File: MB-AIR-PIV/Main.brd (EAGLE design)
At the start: 50.8 x 32.7 mm, 24 parts, among them IC1 MEGA8-AI, IC2 LM1117DTX-5.0, Y1 16MHZ

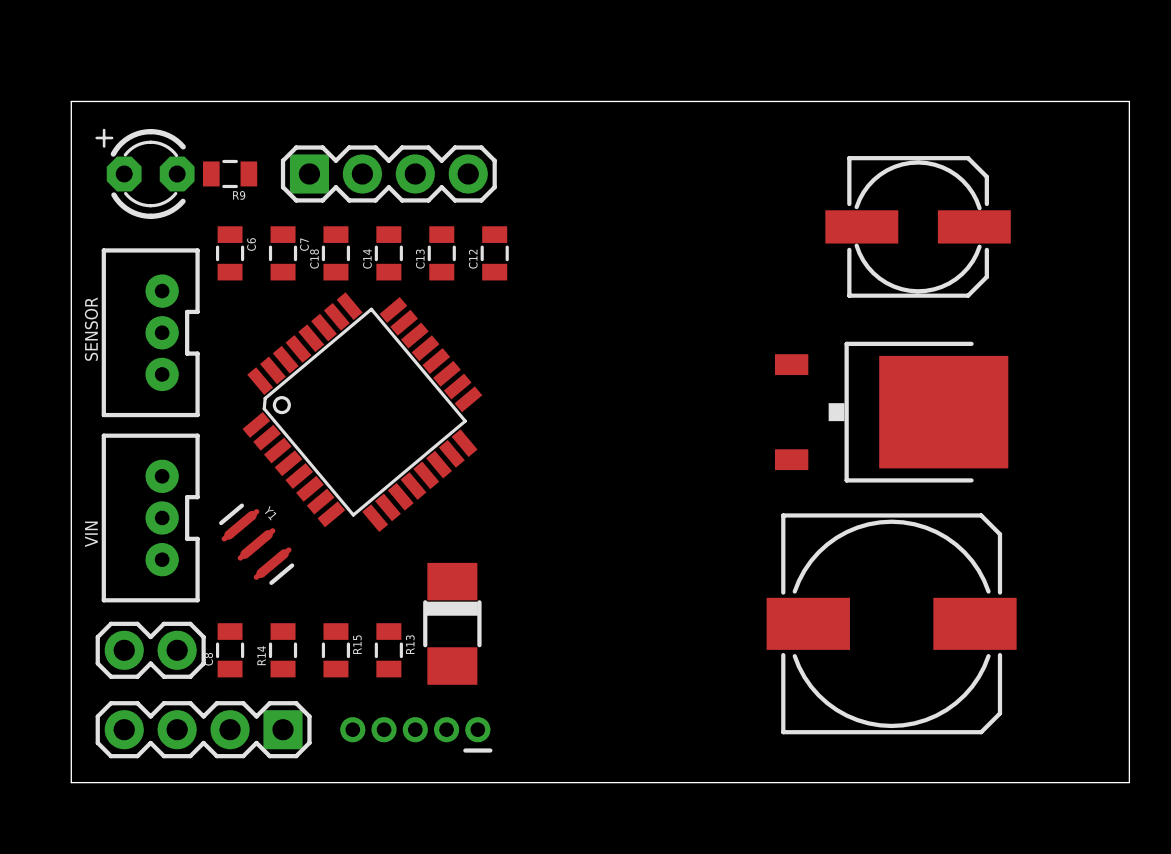
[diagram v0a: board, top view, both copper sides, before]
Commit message: update
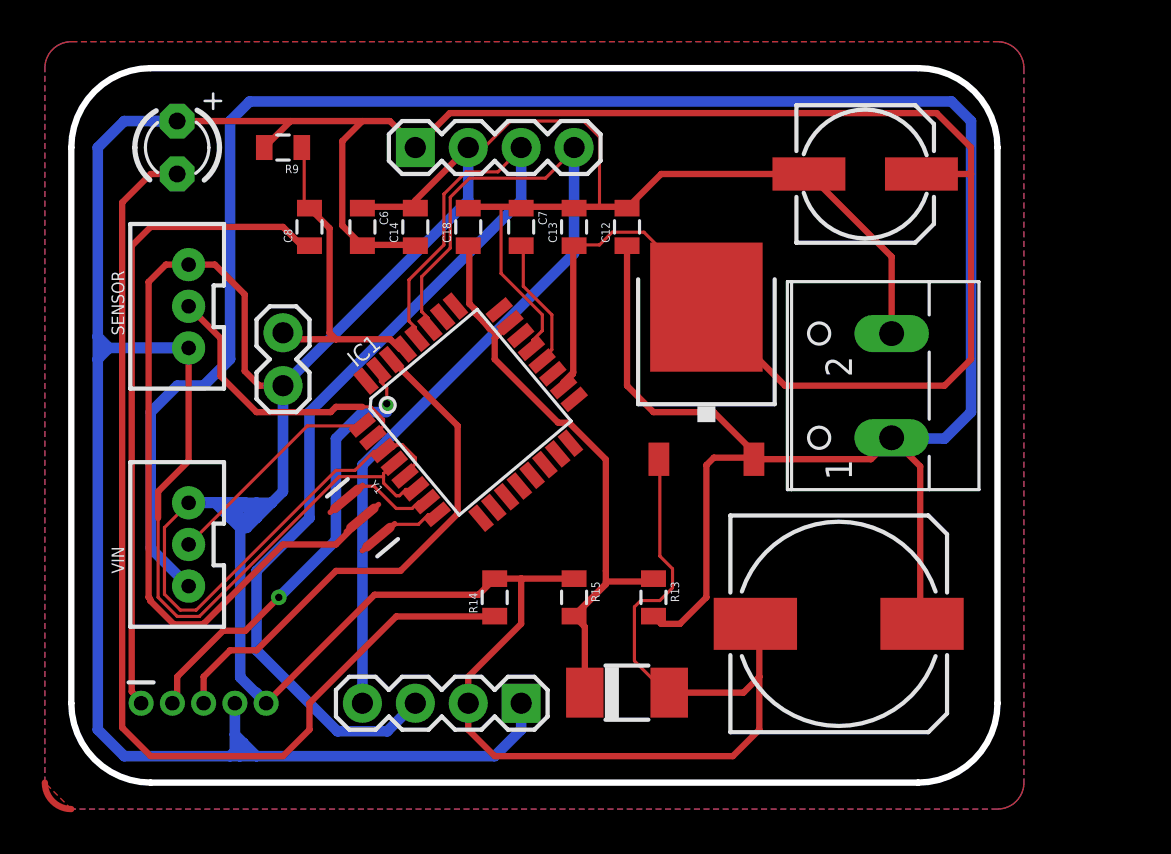
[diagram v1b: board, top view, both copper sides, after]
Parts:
- added X3: RELAY1, con-wago-500:W237-102
- moved C8 20.7 mm to (11.4, 26.7)
- moved JP1 17.0 mm to (10.2, 21.6), turned to 270 degrees
- moved R13 13.0 mm to (27.9, 8.89)
- moved R15 11.7 mm to (24.1, 8.89)
- moved BME280 11.5 mm to (21.6, 3.81)
- moved C7 11.5 mm to (21.6, 26.7)
- moved R14 10.5 mm to (20.3, 8.89)
- moved UPLOAD 10.2 mm to (6.35, 3.81), turned to 0 degrees
- moved IC2 9.25 mm to (30.5, 20.3), turned to 0 degrees
- moved D4 9.01 mm to (26.7, 4.32), turned to 0 degrees
- moved C12 6.48 mm to (26.7, 26.7)
- moved C18 6.48 mm to (19.1, 26.7)
- moved C6 6.48 mm to (14.0, 26.7)
- moved C13 6.48 mm to (24.1, 26.7)
- moved OLED 5.24 mm to (16.5, 30.5)
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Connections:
- net 12V: now also X3.1
- net GND: now also X3.2
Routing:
- net GND: track 0.00 -> 251.6 mm
- net VCC: track 0.00 -> 206.6 mm
- net 12V: track 0.00 -> 140.1 mm
- net SCL: track 0.00 -> 51.7 mm
- net N$12: track 0.00 -> 50.4 mm
- net SDA: track 0.00 -> 44.9 mm
- net A0: track 0.00 -> 31.6 mm
- net N$9: track 0.00 -> 31.5 mm
- net RXD: track 0.00 -> 25.4 mm
- net TXD: track 0.00 -> 21.7 mm, vias 0 -> 2
- net RST: track 0.00 -> 16.6 mm
- net D4: track 0.00 -> 14.0 mm
- net D3: track 0.00 -> 10.7 mm
- net N$8: track 0.00 -> 6.33 mm
- net N$7: track 0.00 -> 4.61 mm
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- added copper zone on layer 16, net B
- added copper zone on layer 1, net T
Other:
- board size 50.8 x 32.7 mm -> 44.5 x 34.3 mm
